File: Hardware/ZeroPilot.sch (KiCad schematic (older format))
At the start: 12 parts, among them J1 CONN_01X03, J2 CONN_01X04

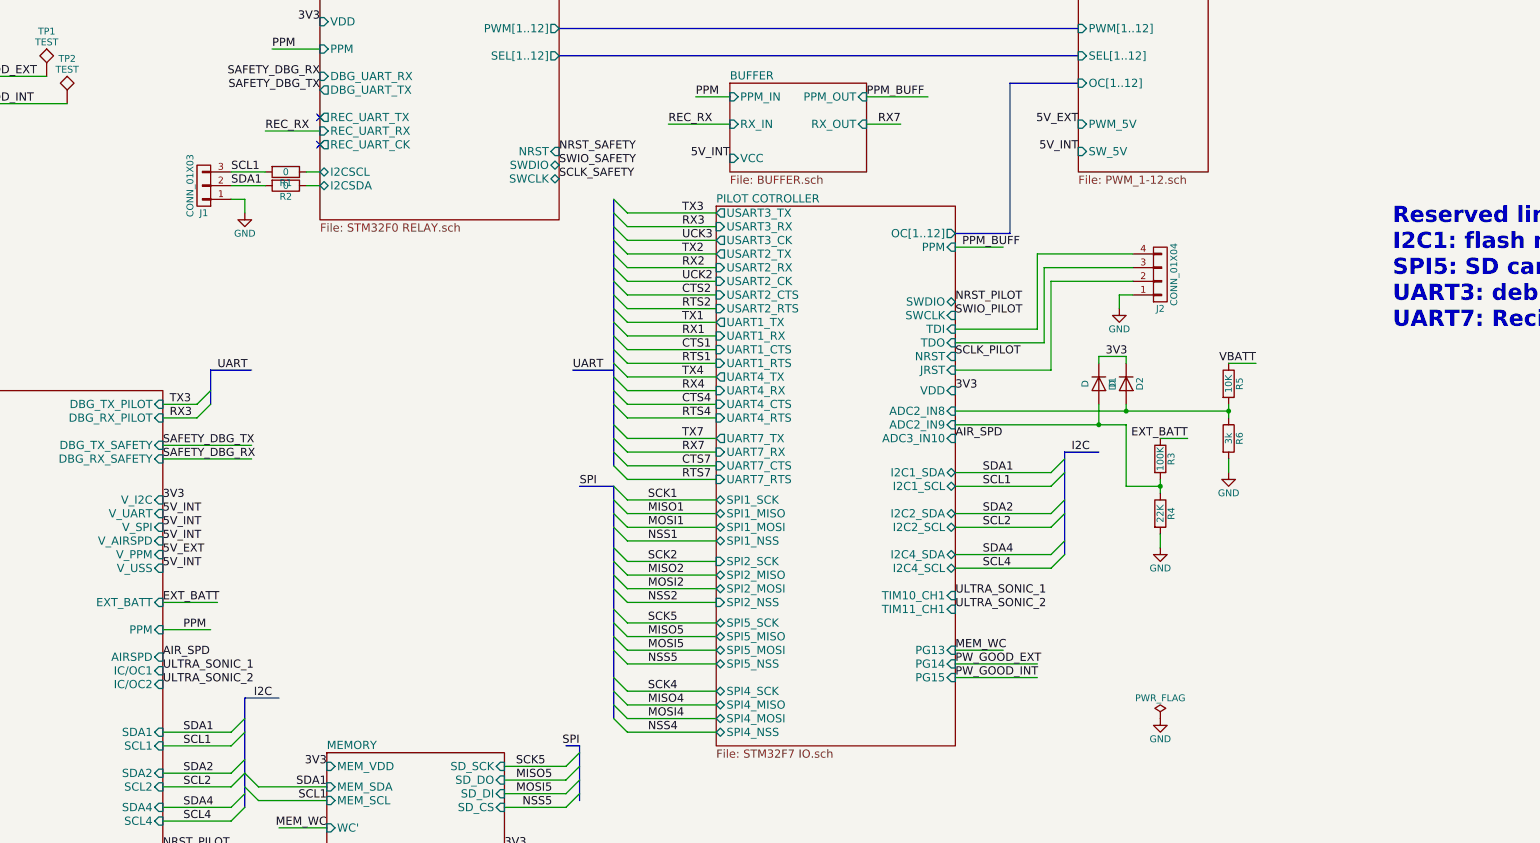
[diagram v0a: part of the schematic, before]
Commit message: Fixed serge suggestions
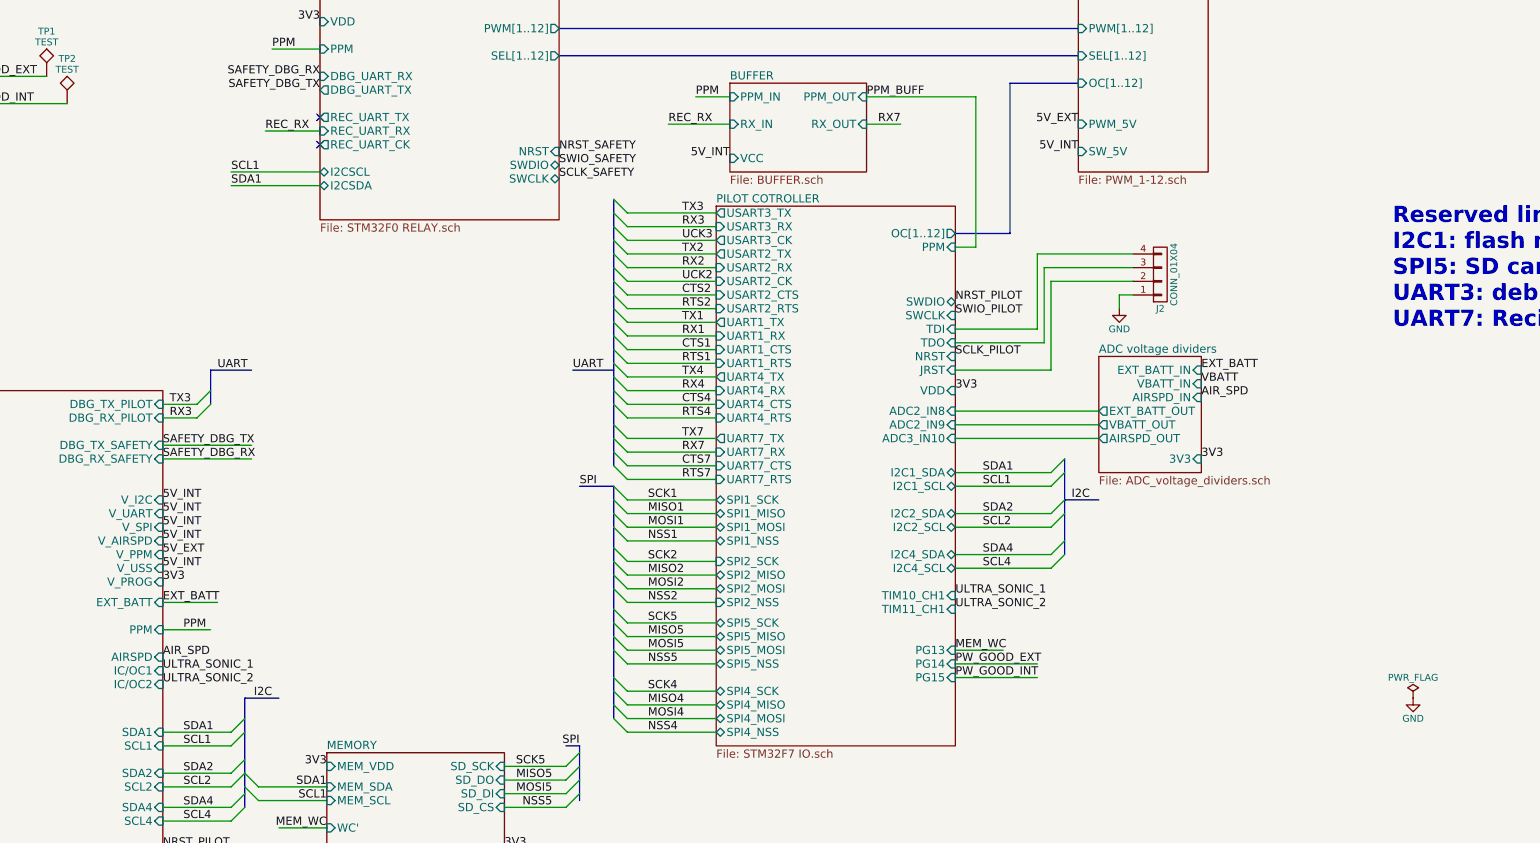
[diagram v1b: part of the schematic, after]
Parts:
- removed D1, D2: D, Diodes_SMD:D_SOD-523, symbol D
- removed J1: CONN_01X03, Pin_Headers:Pin_Header_Straight_1x03_Pitch2.54mm, symbol CONN_01X03
- removed R1, R2: 0, Resistors_SMD:R_0603_HandSoldering, symbol R
- removed R3: 100K, Resistors_SMD:R_0603_HandSoldering, symbol R
- removed R4: 22K, Resistors_SMD:R_0603_HandSoldering, symbol R
- removed R5: 10K, Resistors_SMD:R_0603_HandSoldering, symbol R
- removed R6: 3k, Resistors_SMD:R_0603_HandSoldering, symbol R
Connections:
- wire segments 139 -> 124

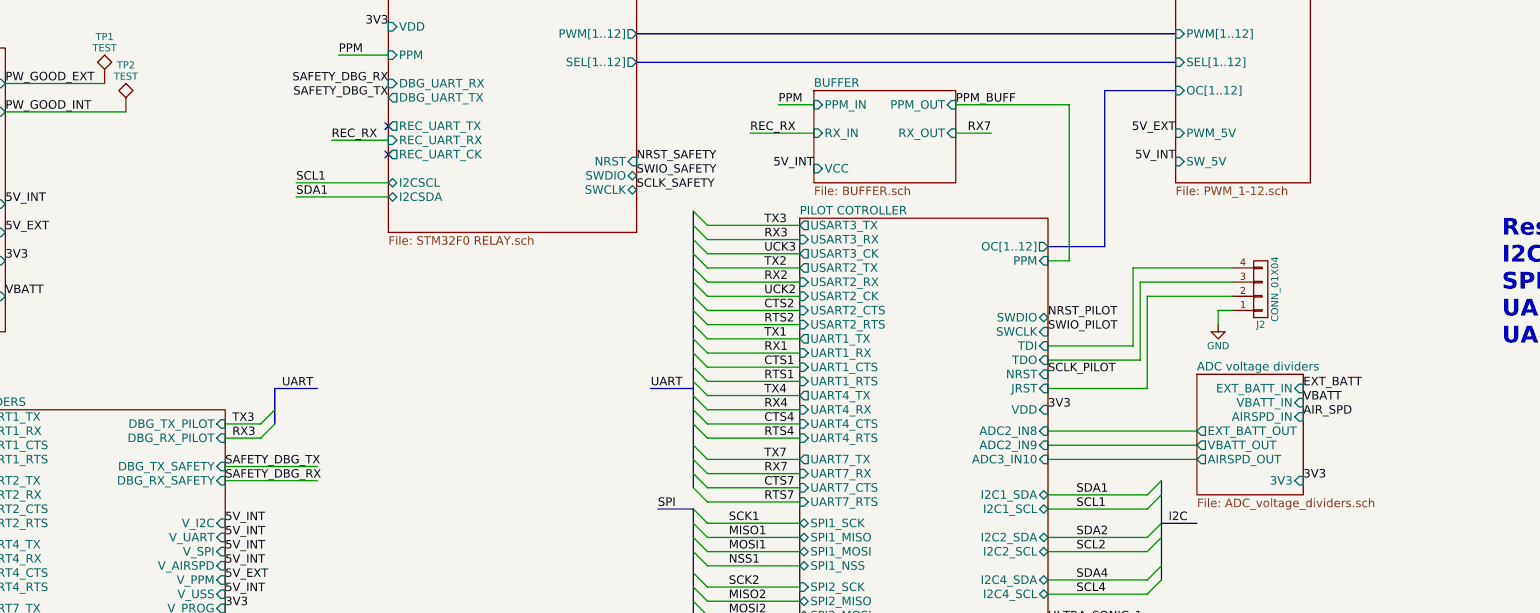
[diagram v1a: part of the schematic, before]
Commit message: commit before my computer restarts
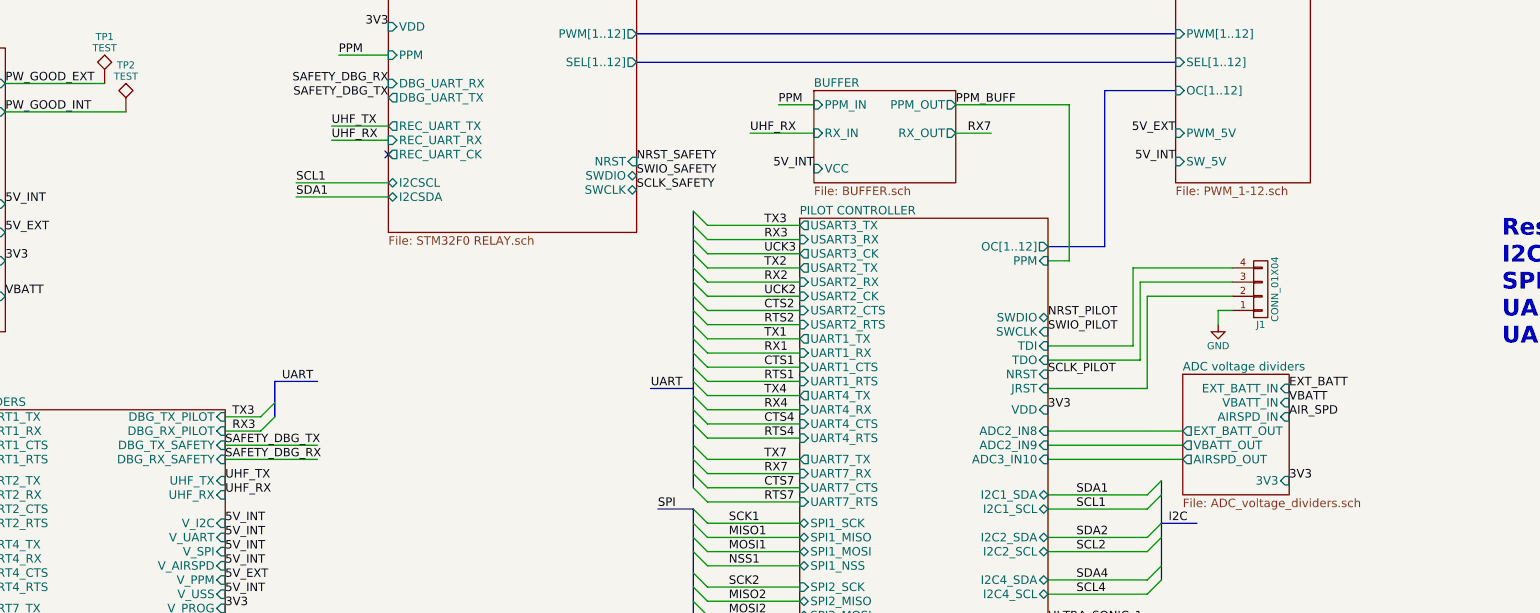
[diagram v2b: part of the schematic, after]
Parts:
- renumbered J2 to J1
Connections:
- net labels added: UHF_RX, UHF_TX
- net labels removed: REC_RX
- wire segments 124 -> 125
- no-connect marks 2 -> 1
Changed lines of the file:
@@
 encoding utf-8
 Sheet 1 21
-Title "Overall Strcture"
+Title "ZeroPilot Overview"
 Date "2017-05-14"
 Rev ""
@@
 F1 "HEADERS.sch" 60
 F2 "EXT_BATT" I R 3150 5150 60
-F3 "DBG_RX_SAFETY" I R 3150 4100 60
-F4 "DBG_TX_SAFETY" I R 3150 4000 60
+F3 "DBG_RX_SAFETY" I R 3150 3950 60
+F4 "DBG_TX_SAFETY" I R 3150 3850 60
 F5 "V_I2C" I R 3150 4400 60
 F6 "SDA1" I R 3150 6100 60
@@
 F53 "UART2_RX" I L 1350 4200 60
 F54 "UART2_CTS" I L 1350 4300 60
-F55 "DBG_RX_PILOT" I R 3150 3800 60
-F56 "DBG_TX_PILOT" I R 3150 3700 60
+F55 "DBG_RX_PILOT" I R 3150 3750 60
+F56 "DBG_TX_PILOT" I R 3150 3650 60
 F57 "NRST_PILOT" I R 3150 6950 60
 F58 "SWIO_PILOT" I R 3150 7050 60
@@
 F62 "SCLK_SAFETY" I R 3150 7500 60
 F63 "V_PROG" I R 3150 5000 60
+F64 "UHF_RX" I R 3150 4200 60
+F65 "UHF_TX" I R 3150 4100 60
 $EndSheet
 $Sheet
 S 7200 2250 1750 3950
 U 5918F046
-F0 "PILOT COTROLLER" 60
+F0 "PILOT CONTROLLER" 60
 F1 "STM32F7 IO.sch" 60
 F2 "PPM" I R 8950 2550 60
@@
 F1 "BUFFER.sch" 60
 F2 "PPM_IN" I L 7300 1450 60
-F3 "PPM_OUT" I R 8300 1450 60
-F4 "VCC" I L 7300 1900 60
-F5 "RX_IN" I L 7300 1650 60
-F6 "RX_OUT" I R 8300 1650 60
+F3 "VCC" I L 7300 1900 60
+F4 "RX_IN" I L 7300 1650 60
+F5 "PPM_OUT" O R 8300 1450 60
+F6 "RX_OUT" O R 8300 1650 60
 $EndSheet
 Text Label 7300 1900 2    60   ~ 0
@@
 Text Label 8300 1450 0    60   ~ 0
 PPM_BUFF
-Text Label 6850 1650 0    60   ~ 0
-REC_RX
 Text Label 8550 1650 2    60   ~ 0
 RX7
 Text Label 3900 1700 0    60   ~ 0
-REC_RX
+UHF_RX
 Entry Wire Line
 	6450 2700 6550 2800
@@
 Text Label 950  5550 0    59   ~ 0
 UCK2
-Text Label 3550 3450 0    59   ~ 0
+Text Label 3550 3400 0    59   ~ 0
 UART
 Entry Wire Line
-	3400 3700 3500 3600
-Entry Wire Line
-	3400 3800 3500 3700
-Text Label 3200 3700 0    59   ~ 0
+	3400 3650 3500 3550
+Entry Wire Line
+	3400 3750 3500 3650
+Text Label 3200 3650 0    59   ~ 0
 TX3
-Text Label 3200 3800 0    59   ~ 0
+Text Label 3200 3750 0    59   ~ 0
 RX3
 Text Label 4300 1300 2    59   ~ 0
 SAFETY_DBG_RX
-Text Label 3150 4100 0    59   ~ 0
+Text Label 3150 3950 0    59   ~ 0
 SAFETY_DBG_RX
 Text Label 4300 1400 2    59   ~ 0
 SAFETY_DBG_TX
-Text Label 3150 4000 0    59   ~ 0
+Text Label 3150 3850 0    59   ~ 0
 SAFETY_DBG_TX
 Text Label 650  5650 0    60   ~ 0
@@
 	1350 5550 700  5550
 Wire Bus Line
-	3500 3450 3500 3700
-Wire Bus Line
-	3500 3450 3800 3450
-Wire Wire Line
-	3400 3800 3150 3800
-Wire Wire Line
-	3150 3700 3400 3700
-Wire Wire Line
-	3150 4000 3800 4000
-Wire Wire Line
-	3150 4100 3800 4100
+	3500 3400 3500 3650
+Wire Bus Line
+	3500 3400 3800 3400
+Wire Wire Line
+	3400 3750 3150 3750
+Wire Wire Line
+	3150 3650 3400 3650
+Wire Wire Line
+	3150 3850 3800 3850
+Wire Wire Line
+	3150 3950 3800 3950
 Wire Bus Line
 	600  5650 600  7350
@@
 SCLK_SAFETY
 $Comp
-L CONN_01X04 J2
+L CONN_01X04 J1
 U 1 1 594DE28B
 P 10450 2750
-F 0 "J2" H 10450 3000 50  0000 C CNN
+F 0 "J1" H 10450 3000 50  0000 C CNN
 F 1 "CONN_01X04" V 10550 2750 50  0000 C CNN
 F 2 "Pin_Headers:Pin_Header_Straight_1x04_Pitch2.54mm" H 10450 2750 50  0001 C CNN
@@
 	1    0    0    -1
 $EndComp
-NoConn ~ 4300 1600
 NoConn ~ 4300 1800
 Text Label 5650 6950 0    60   ~ 0
@@
 3V3
 $Sheet
-S 10000 3350 750  850
+S 9900 3350 750  850
 U 59688A25
 F0 "ADC voltage dividers" 60
 F1 "ADC_voltage_dividers.sch" 60
-F2 "EXT_BATT_IN" I R 10750 3450 60
-F3 "EXT_BATT_OUT" O L 10000 3750 60
-F4 "VBATT_IN" I R 10750 3550 60
-F5 "VBATT_OUT" O L 10000 3850 60
-F6 "AIRSPD_IN" I R 10750 3650 60
-F7 "3V3" I R 10750 4100 60
-F8 "AIRSPD_OUT" O L 10000 3950 60
+F2 "EXT_BATT_IN" I R 10650 3450 60
+F3 "EXT_BATT_OUT" O L 9900 3750 60
+F4 "VBATT_IN" I R 10650 3550 60
+F5 "VBATT_OUT" O L 9900 3850 60
+F6 "AIRSPD_IN" I R 10650 3650 60
+F7 "3V3" I R 10650 4100 60
+F8 "AIRSPD_OUT" O L 9900 3950 60
 $EndSheet
 Wire Wire Line
-	10000 3950 8950 3950
-Wire Wire Line
-	8950 3850 10000 3850
-Wire Wire Line
-	10000 3750 8950 3750
-Text Label 10750 4100 0    60   ~ 0
+	9900 3950 8950 3950
+Wire Wire Line
+	8950 3850 9900 3850
+Wire Wire Line
+	9900 3750 8950 3750
+Text Label 10650 4100 0    60   ~ 0
 3V3
-Text Label 10750 3650 0    60   ~ 0
+Text Label 10650 3650 0    60   ~ 0
 AIR_SPD
-Text Label 10750 3550 0    60   ~ 0
+Text Label 10650 3550 0    60   ~ 0
 VBATT
-Text Label 10750 3450 0    60   ~ 0
+Text Label 10650 3450 0    60   ~ 0
 EXT_BATT
+Wire Wire Line
+	4300 1600 3900 1600
+Text Label 3900 1600 0    60   ~ 0
+UHF_TX
+Text Label 3150 4100 0    60   ~ 0
+UHF_TX
+Text Label 3150 4200 0    60   ~ 0
+UHF_RX
+Text Label 6850 1650 0    60   ~ 0
+UHF_RX
 $EndSCHEMATC
